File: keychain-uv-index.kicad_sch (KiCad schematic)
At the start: 16 parts, among them J1 Conn_01x06_Pin, SW1 SW_Push_Dual, U1 ATtiny85V-10S

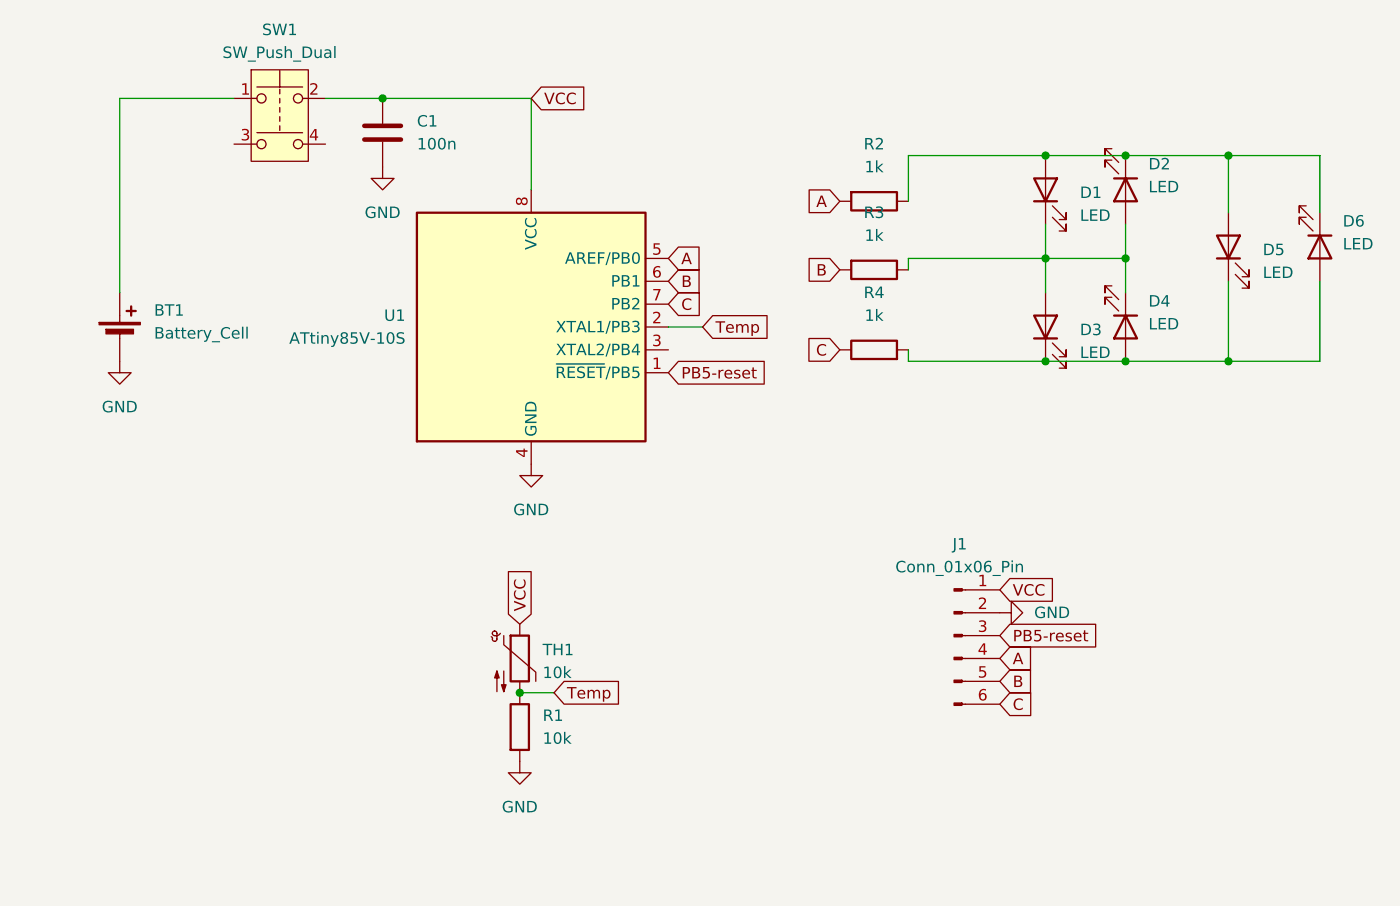
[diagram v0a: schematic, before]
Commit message: edited schematics
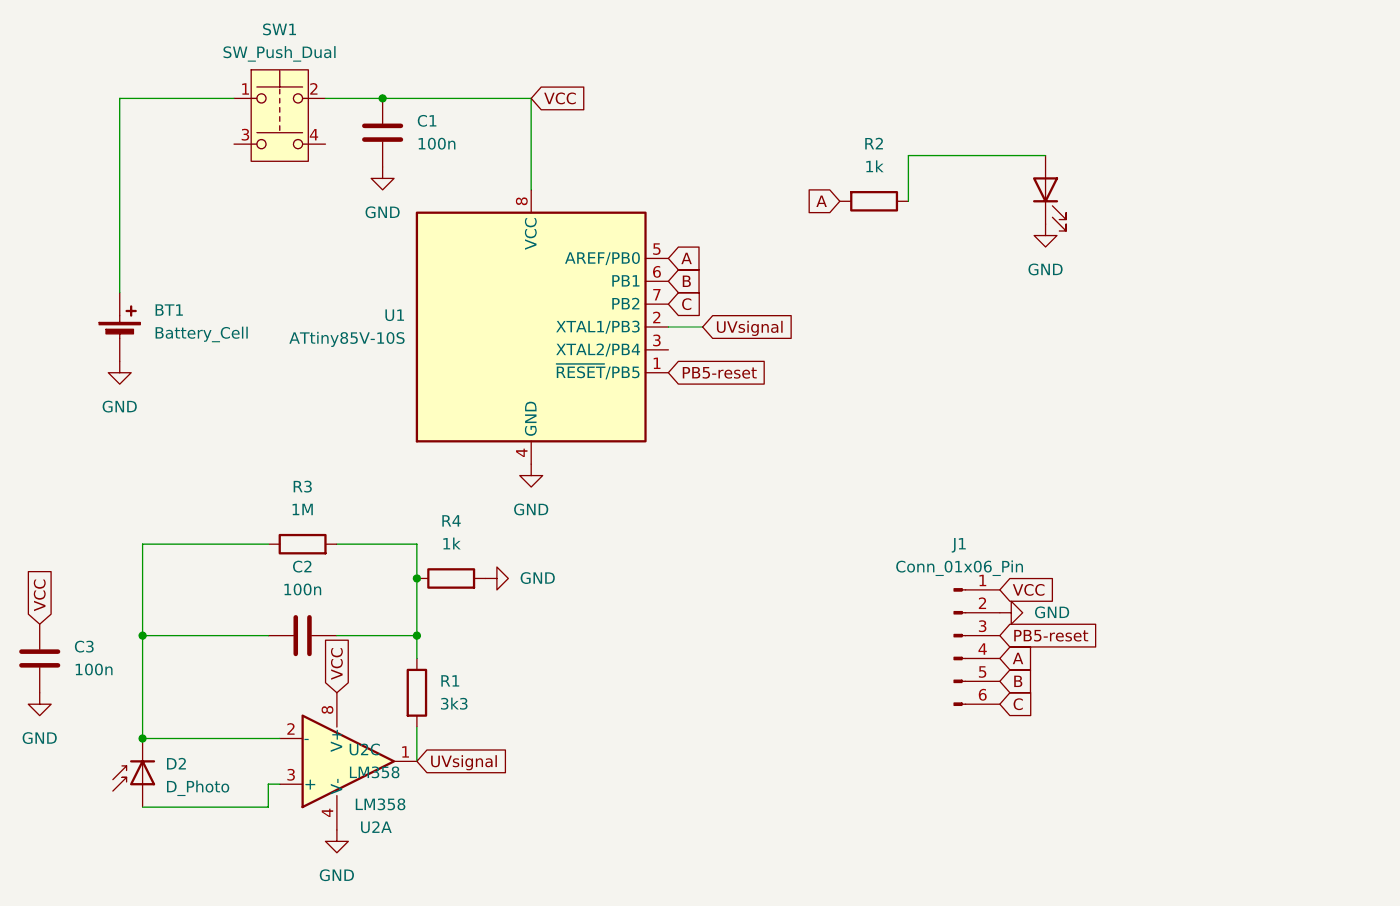
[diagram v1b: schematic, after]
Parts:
- removed D2, D3, D4, D5, D6: LED, LED_SMD:LED_0805_2012Metric, symbol Device:LED
- removed TH1: 10k, Resistor_SMD:R_0805_2012Metric, symbol Device:Thermistor_NTC
- added C2, C3: 100n, Capacitor_SMD:C_0805_2012Metric, symbol Device:C
- added D2: D_Photo, LED_SMD:LED_PLCC-2_3.4x3.0mm_AK, symbol Device:D_Photo
- added U2: LM358, Package_SO:SOIC-8W_5.3x5.3mm_P1.27mm, symbol Amplifier_Operational:LM358
- R1: value 10k -> 3k3
- R3: value 1k -> 1M
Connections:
- net B: no longer R3.2
- net C: no longer R4.1
- net GND: now also D1.1 (K), R4.2, C3.1, U2.4 (V-); no longer R1.2
- net VCC: now also C3.2, U2.8 (V+)
- net at R3.1: now also C2.1, D2.1 (K), U2.2 (-); no longer D1.1 (K)
- net Temp: no longer names the net of R1.1
- net Temp: now also R3.2, R4.1, C2.2; no longer U1.2 (XTAL1/PB3)
- new net: D2.2 (A), U2.3 (+)
- new net UVsignal: R1.2, U1.2 (XTAL1/PB3), U2.1
